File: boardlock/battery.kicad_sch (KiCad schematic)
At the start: 18 parts, among them J2 Conn_01x02_MountingPin, U4 BQ27441DRZR-G1A, U5 BQ24075RGT

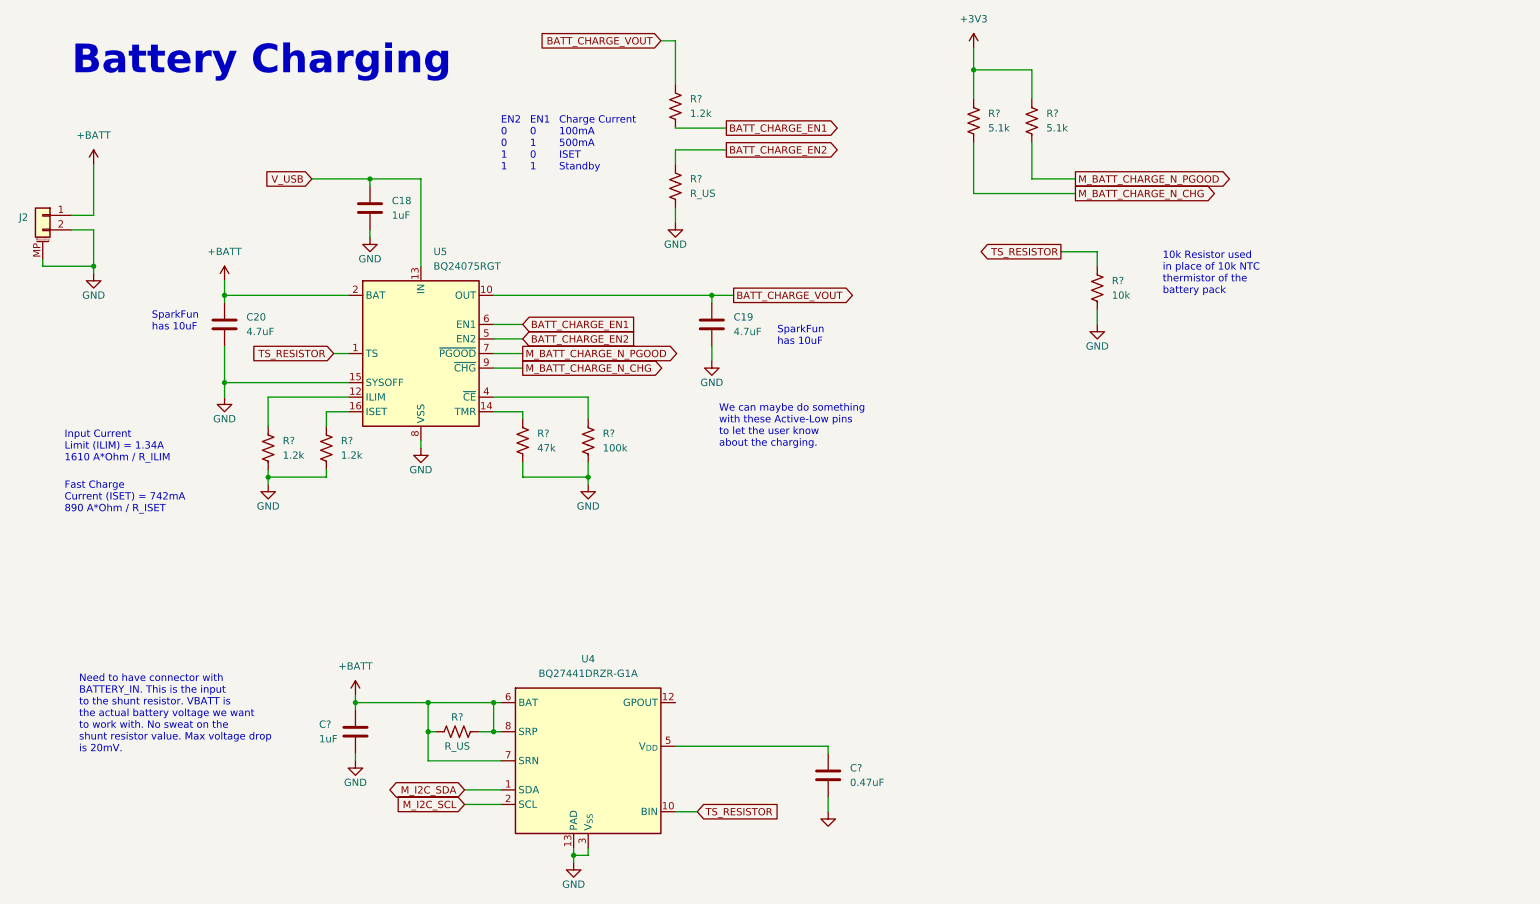
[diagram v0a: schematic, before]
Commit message: finishing touches
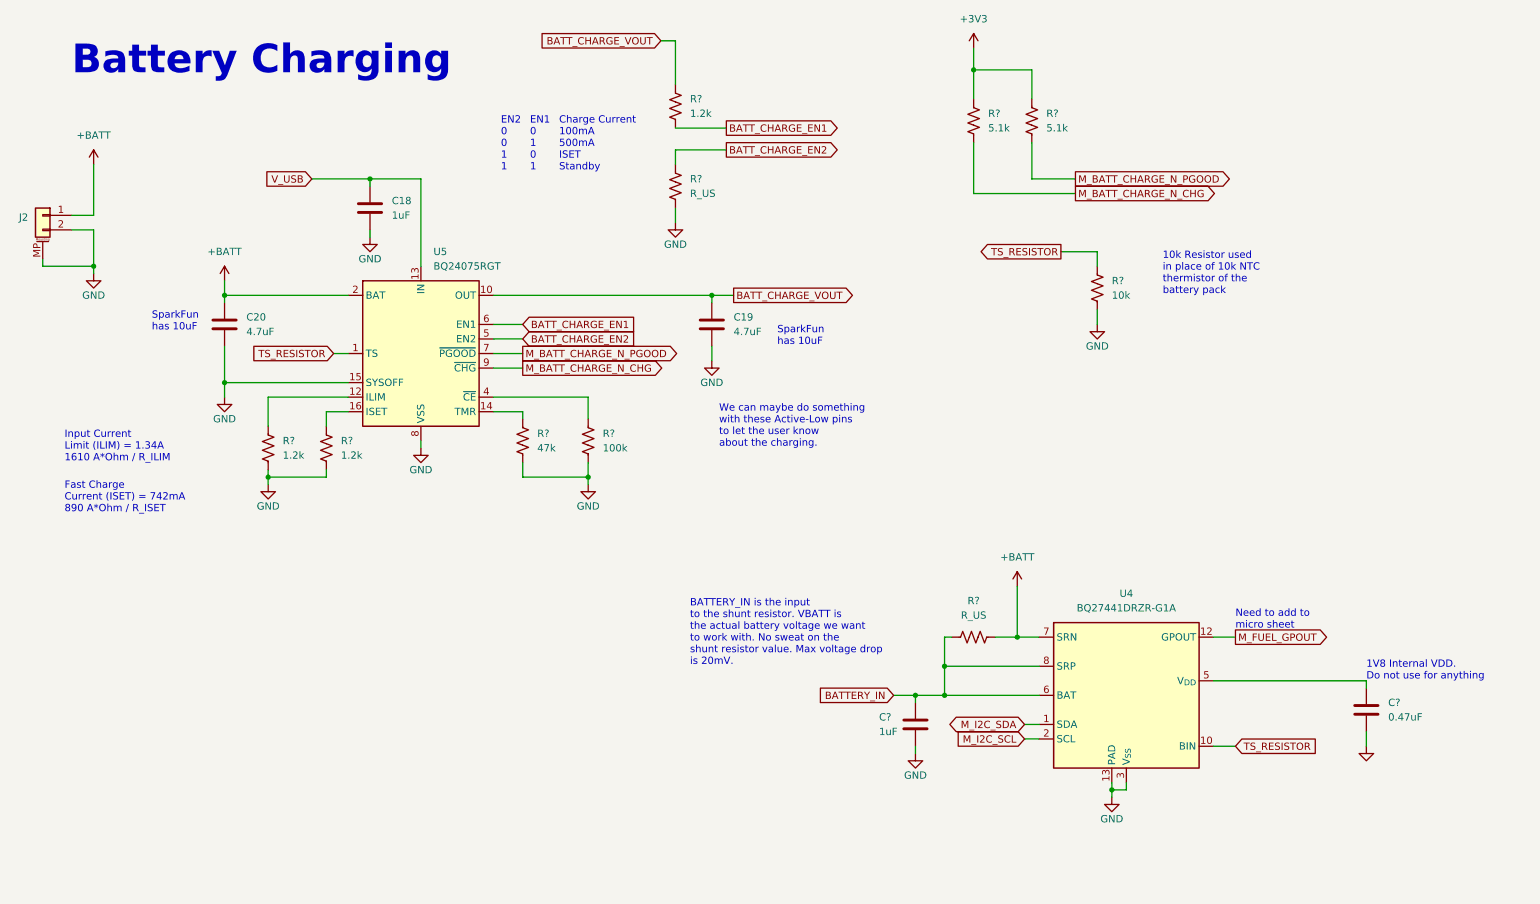
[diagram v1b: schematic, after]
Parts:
- removed R?: R_US, symbol Device:R_US
- added R?: R_US, symbol Device:R_US
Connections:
- net +BATT: now also R?.1; no longer C?.1, U4.6 (BAT), U4.8 (SRP)
- net M_FUEL_GPOUT: now reaches U4.12 (GPOUT)
- new net BATTERY_IN: C?.1, R?.2, U4.6 (BAT), U4.8 (SRP)
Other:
- note added: "1V8 Internal VDD. Do not use for anything"
- note added: "BATTERY_IN is the input to the shunt resistor. VBATT is the actual battery voltage we want to work with. No sweat on the shunt resistor value. Max voltage drop is 20mV."
- note added: "Need to add to micro sheet"
- note removed: "Need to have connector with BATTERY_IN. This is the input to the shunt resistor. VBATT is the actual battery voltage we want to work with. No sweat on the shunt resistor value. Max voltage drop is 20mV."
- moved on the sheet: C?, U4
